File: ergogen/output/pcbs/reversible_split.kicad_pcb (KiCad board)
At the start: 2 copper layers, 141.4 x 97.7 mm, 22 parts

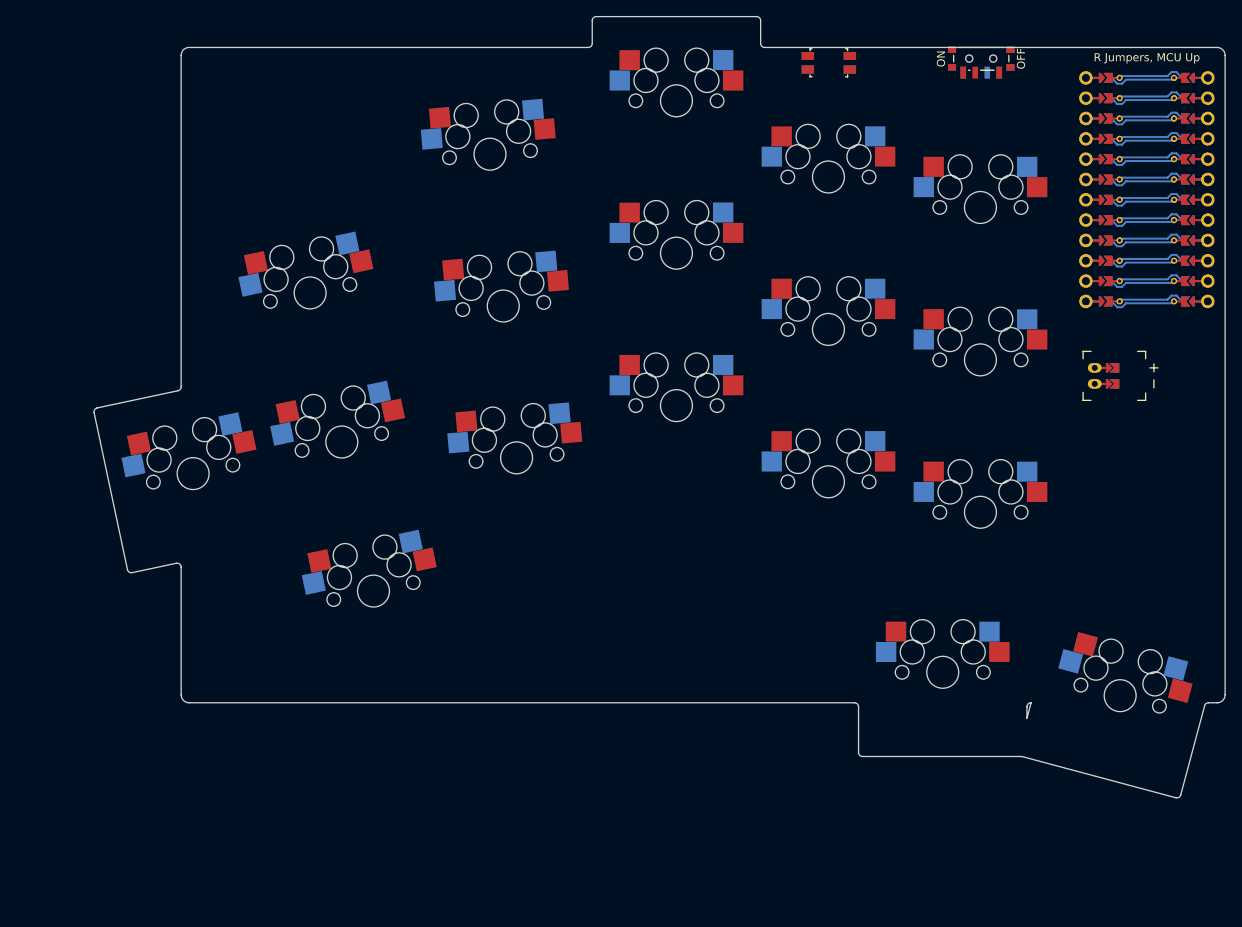
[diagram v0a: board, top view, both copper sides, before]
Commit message: Rotated layout experiment
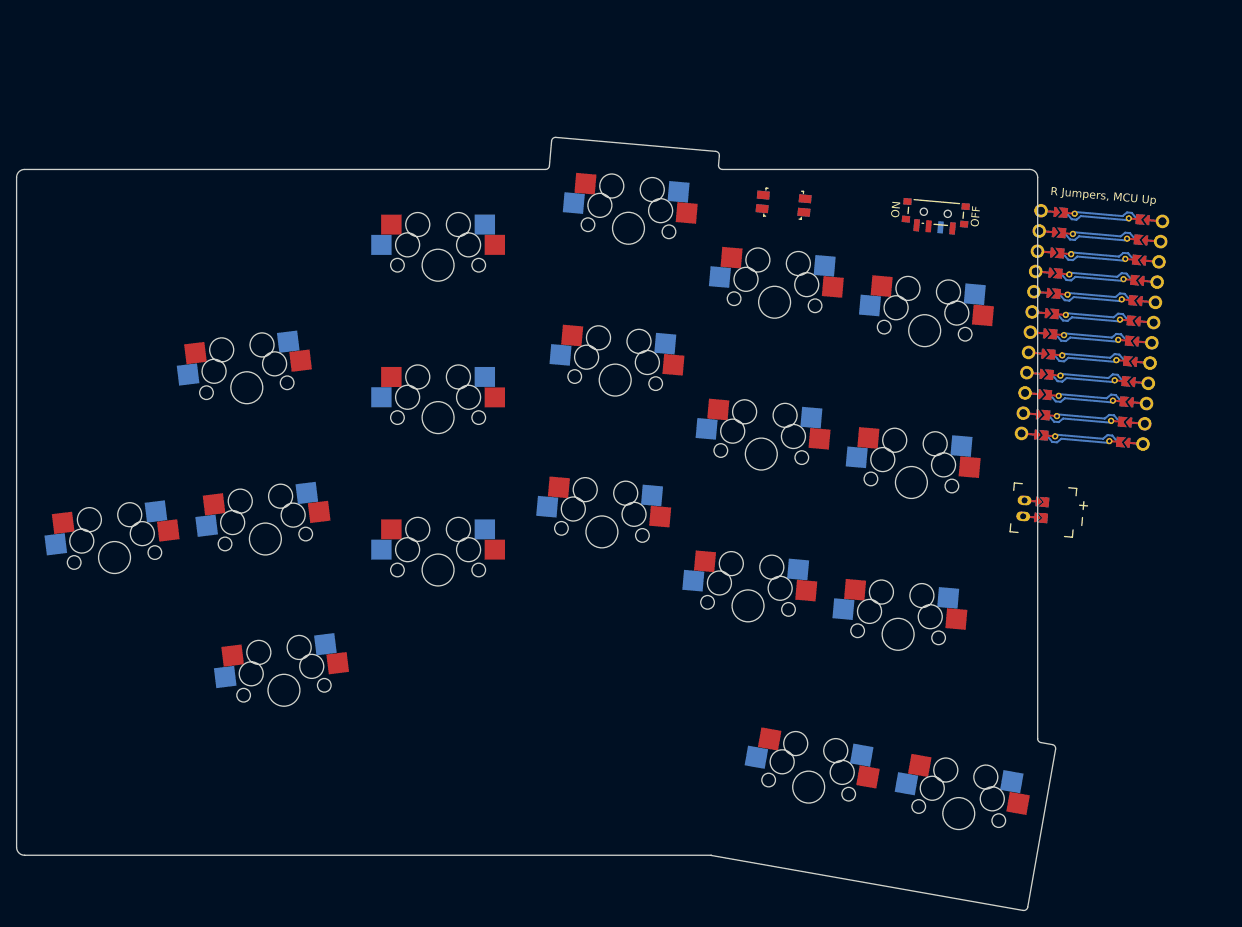
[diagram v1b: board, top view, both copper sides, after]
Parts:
- moved S18 25.0 mm to (220.7, 149.8), turned to -10 degrees
- moved S17 22.1 mm to (202.0, 146.5), turned to -10 degrees
- moved PWR1 20.1 mm to (217.9, 74.7), turned to 85 degrees
- moved JST1 18.8 mm to (228.9, 111.6), turned to 85 degrees
- moved MCU1 18.5 mm to (237.5, 87.8), turned to -5 degrees
- moved RST1 18.5 mm to (198.9, 73.6), turned to -5 degrees
- moved S11 18.5 mm to (194.4, 123.8), turned to -5 degrees
- moved S14 18.4 mm to (213.2, 127.4), turned to -5 degrees
- moved S8 18.3 mm to (176.1, 114.6), turned to -5 degrees
- moved S12 17.7 mm to (196.1, 104.9), turned to -5 degrees
- moved S9 17.6 mm to (177.8, 95.6), turned to -5 degrees
- moved S15 17.6 mm to (214.8, 108.4), turned to -5 degrees
- moved S5 17.1 mm to (155.7, 119.3), turned to 0 degrees
- moved S13 17.0 mm to (197.7, 85.9), turned to -5 degrees
- moved S10 17.0 mm to (179.5, 76.6), turned to -5 degrees
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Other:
- board size 141.4 x 97.7 mm -> 129.9 x 96.6 mm
